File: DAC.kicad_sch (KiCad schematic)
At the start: 2 parts, among them U3 LM741

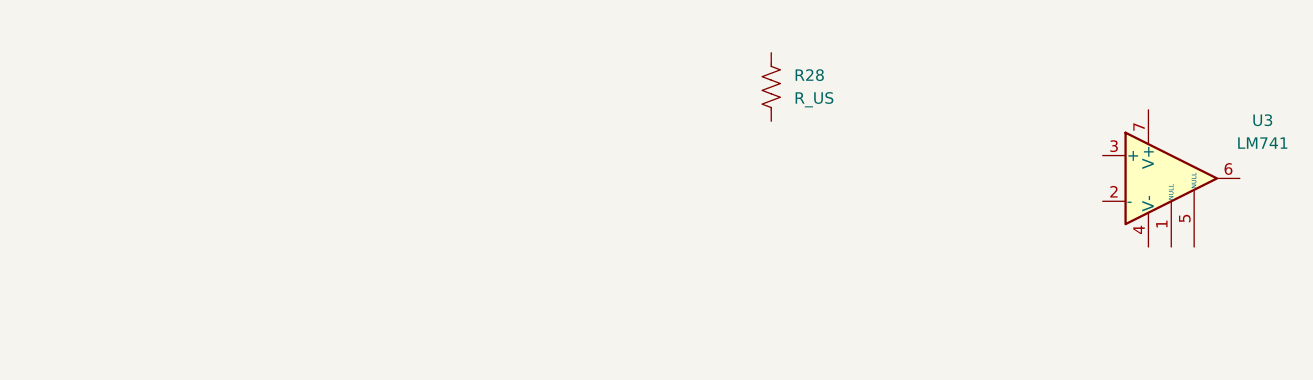
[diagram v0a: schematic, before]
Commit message: Edited DAC
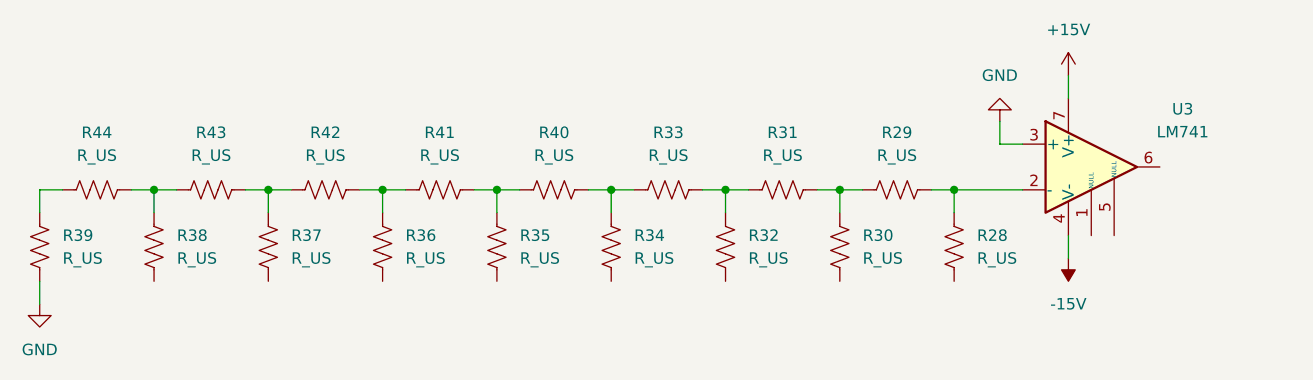
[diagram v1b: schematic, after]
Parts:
- added R29, R30, R31, R32, R33, R34, R35, R36, R37, R38, R39, R40, R41, R42, R43, R44: R_US, Resistor_THT:R_Axial_DIN0207_L6.3mm_D2.5mm_P10.16mm_Horizontal, symbol Device:R_US
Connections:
- net at R28.1: now also U3.2 (-), R29.1
- net GND: now reaches U3.3 (+)
- net GND: now also R39.2
- net -15V: now reaches U3.4 (V-)
- net +15V: now reaches U3.7 (V+)
- new net: R31.2, R32.1, R33.1
- new net: R33.2, R34.1, R40.1
- new net: R36.1, R41.2, R42.1
- new net: R35.1, R40.2, R41.1
- new net: R37.1, R42.2, R43.1
- new net: R38.1, R43.2, R44.1
- new net: R29.2, R30.1, R31.1
- new net: R39.1, R44.2
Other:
- moved on the sheet: R28, U3
